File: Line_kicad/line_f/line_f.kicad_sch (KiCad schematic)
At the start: 15 parts, among them M2 Motor_DC, M3 Motor_DC, SW1 SW_SPST, SW2 SW_SPDT, SW3 SW_Push, SW4 SW_Push, U1 TB6612FNG_LINE, m1 BLACKPILL

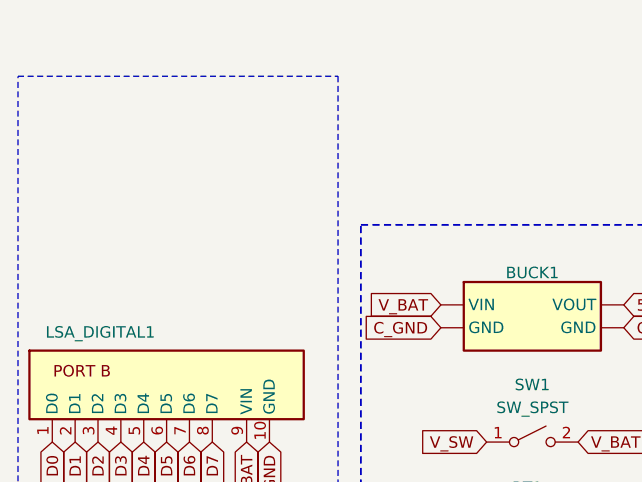
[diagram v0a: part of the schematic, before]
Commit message: 3#
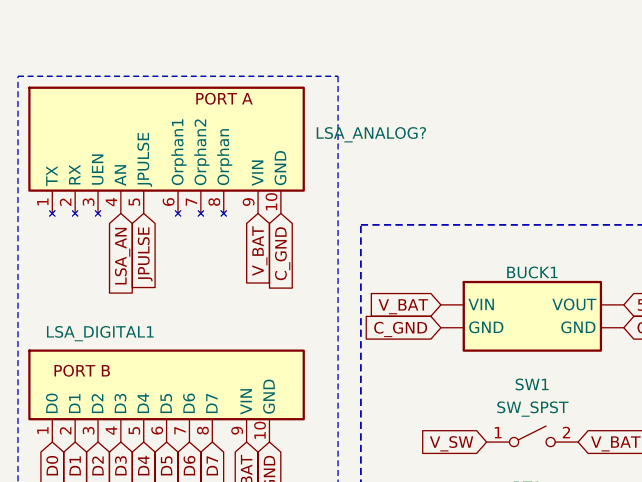
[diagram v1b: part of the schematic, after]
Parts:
- added LSA_ANALOG?: ~, symbol LINE_F_SYM_LIB:LSA_ANALOG
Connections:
- net C_GND: now also LSA_ANALOG?.10 (GND)
- net JPULSE: now also LSA_ANALOG?.5 (JPULSE)
- net LSA_AN: now also LSA_ANALOG?.4 (AN)
- net V_BAT: now also LSA_ANALOG?.9 (VIN)
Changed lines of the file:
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@@
+		)
+	)
+	(global_label "LSA_AN"
+		(shape input)
+		(at 36.83 83.82 270)
+		(fields_autoplaced yes)
+		(effects
+			(font
+				(size 1.27 1.27)
+			)
+			(justify right)
+		)
+		(property "Intersheetrefs" "${INTERSHEET_REFS}"
+			(at 36.83 93.5181 90)
+			(effects
+				(font
+					(size 1.27 1.27)
+				)
+				(justify right)
+				(hide yes)
+			)
+		)
+	)
+	(global_label "V_BAT"
+		(shape input)
+		(at 52.07 83.82 270)
+		(fields_autoplaced yes)
+		(effects
+			(font
+				(size 1.27 1.27)
+			)
+			(justify right)
+		)
+		(property "Intersheetrefs" "${INTERSHEET_REFS}"
+			(at 52.07 92.1876 90)
+			(effects
+				(font
+					(size 1.27 1.27)
+				)
+				(justify right)
+				(hide yes)
+			)
 		)
 	)
@@
 		)
 	)
+	(global_label "C_GND"
+		(shape input)
+		(at 54.61 83.82 270)
+		(fields_autoplaced yes)
+		(effects
+			(font
+				(size 1.27 1.27)
+			)
+			(justify right)
+		)
+		(property "Intersheetrefs" "${INTERSHEET_REFS}"
+			(at 54.61 92.9133 90)
+			(effects
+				(font
+					(size 1.27 1.27)
+				)
+				(justify right)
+				(hide yes)
+			)
+		)
+	)
 	(global_label "PWMA"
 		(shape input)
@@
 		)
 	)
+	(global_label "JPULSE"
+		(shape input)
+		(at 39.37 83.82 270)
+		(fields_autoplaced yes)
+		(effects
+			(font
+				(size 1.27 1.27)
+			)
+			(justify right)
+		)
+		(property "Intersheetrefs" "${INTERSHEET_REFS}"
+			(at 39.37 93.7599 90)
+			(effects
+				(font
+					(size 1.27 1.27)
+				)
+				(justify right)
+				(hide yes)
+			)
+		)
+	)
 	(global_label "D2"
 		(shape input)
@@
 			)
 		)
+	)
+	(symbol
+		(lib_id "LINE_F_SYM_LIB:LSA_ANALOG")
+		(at 41.91 78.74 0)
+		(unit 1)
+		(exclude_from_sim no)
+		(in_bom yes)
+		(on_board yes)
+		(dnp no)
+		(fields_autoplaced yes)
+		(property "Reference" "LSA_ANALOG?"
+			(at 58.42 74.9299 0)
+			(effects
+				(font
+					(size 1.27 1.27)
+				)
+				(justify left)
+			)
+		)
+		(property "Value" "~"
+			(at 58.42 76.835 0)
+			(effects
+				(font
+					(size 1.27 1.27)
+				)
+				(justify left)
+			)
+		)
+		(property "Footprint" ""
+			(at 41.91 78.74 0)
+			(effects
+				(font
+					(size 1.27 1.27)
+				)
+				(hide yes)
+			)
+		)
+		(property "Datasheet" ""
+			(at 41.91 78.74 0)
+			(effects
+				(font
+					(size 1.27 1.27)
+				)
+				(hide yes)
+			)
+		)
+		(property "Description" ""
+			(at 41.91 78.74 0)
+			(effects
+				(font
+					(size 1.27 1.27)
+				)
+				(hide yes)
+			)
+		)
+		(pin "1"
+		)
+		(pin "5"
+		)
+		(pin "9"
+		)
+		(pin "7"
+		)
+		(pin "2"
+		)
+		(pin "10"
+		)
+		(pin "3"
+		)
+		(pin "6"
+		)
+		(pin "4"
+		)
+		(pin "8"
+		)
+		(instances
+			(project ""
+				(path "/c13c4e87-a023-4a7d-8b82-fe1a380f0003"
+					(reference "LSA_ANALOG?")
+					(unit 1)
+				)
+			)
+		)

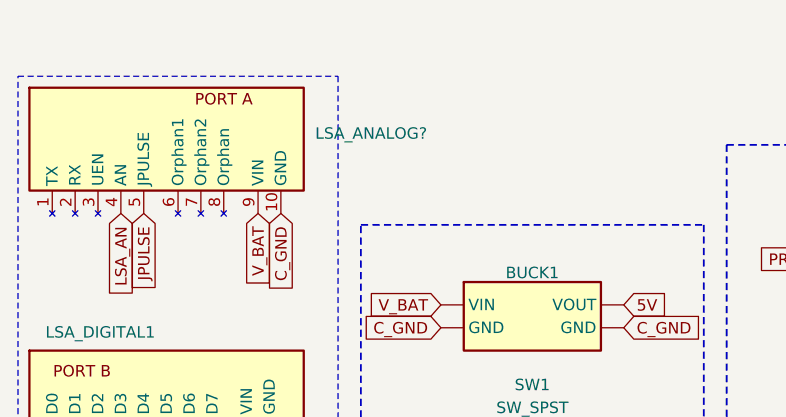
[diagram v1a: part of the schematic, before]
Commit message: 4#
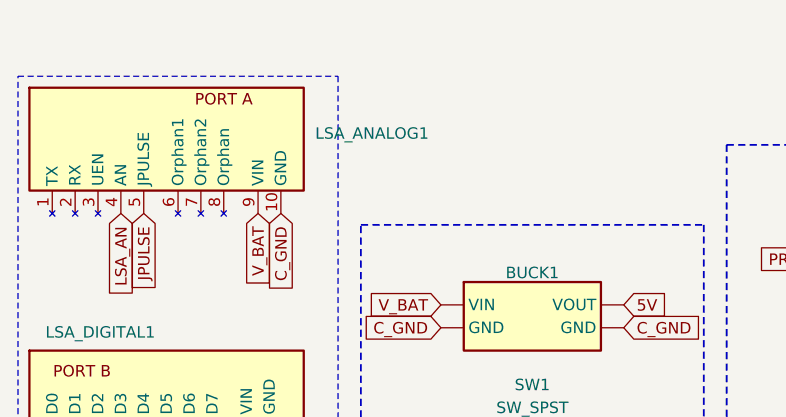
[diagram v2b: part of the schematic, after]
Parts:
- gave numbers to parts that had none: 1
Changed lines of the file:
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@@
 		(dnp no)
 		(fields_autoplaced yes)
-		(property "Reference" "LSA_ANALOG?"
+		(property "Reference" "LSA_ANALOG1"
 			(at 58.42 74.9299 0)
 			(effects
@@
 			(project ""
 				(path "/c13c4e87-a023-4a7d-8b82-fe1a380f0003"
-					(reference "LSA_ANALOG?")
+					(reference "LSA_ANALOG1")
 					(unit 1)
 				)

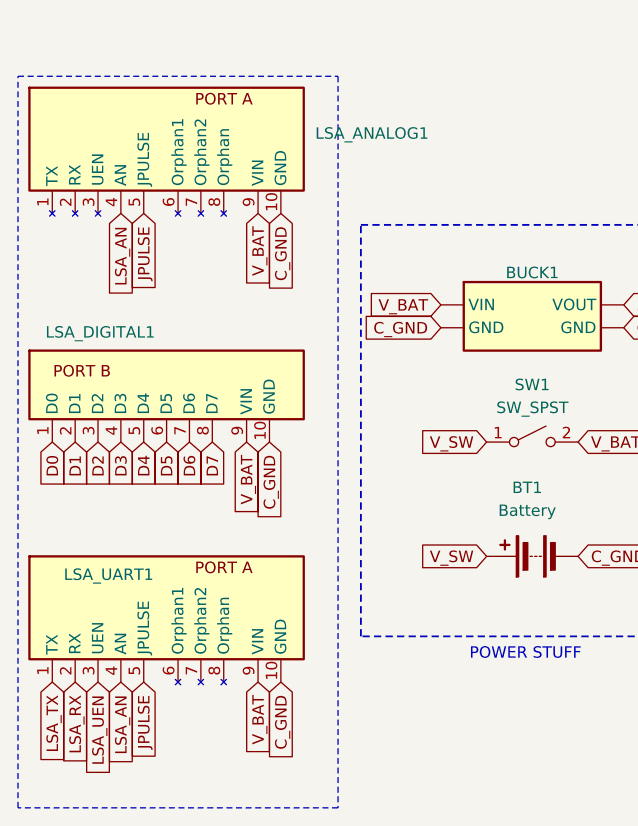
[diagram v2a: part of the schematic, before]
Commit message: 4#
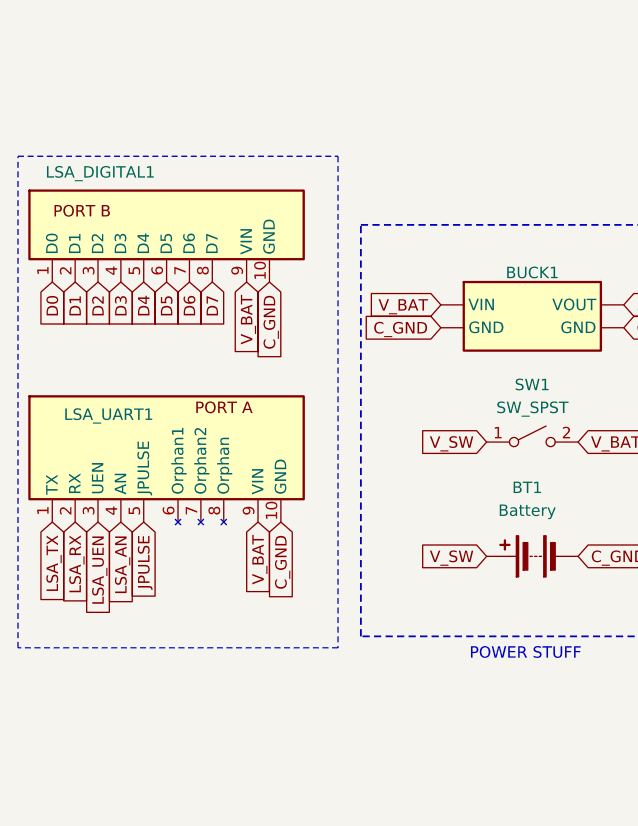
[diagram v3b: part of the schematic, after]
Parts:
- removed LSA_ANALOG1: ~, symbol LINE_F_SYM_LIB:LSA_ANALOG
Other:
- moved on the sheet: LSA_DIGITAL1, LSA_UART1

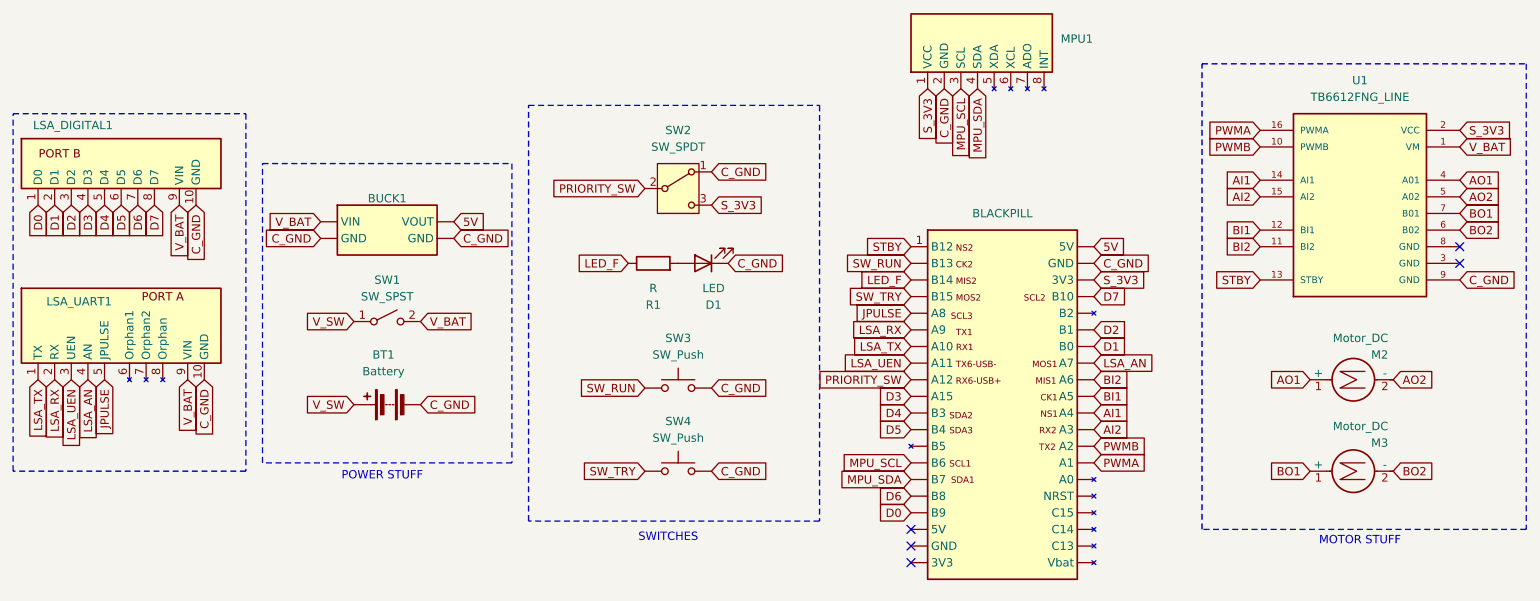
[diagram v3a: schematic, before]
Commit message: 4#
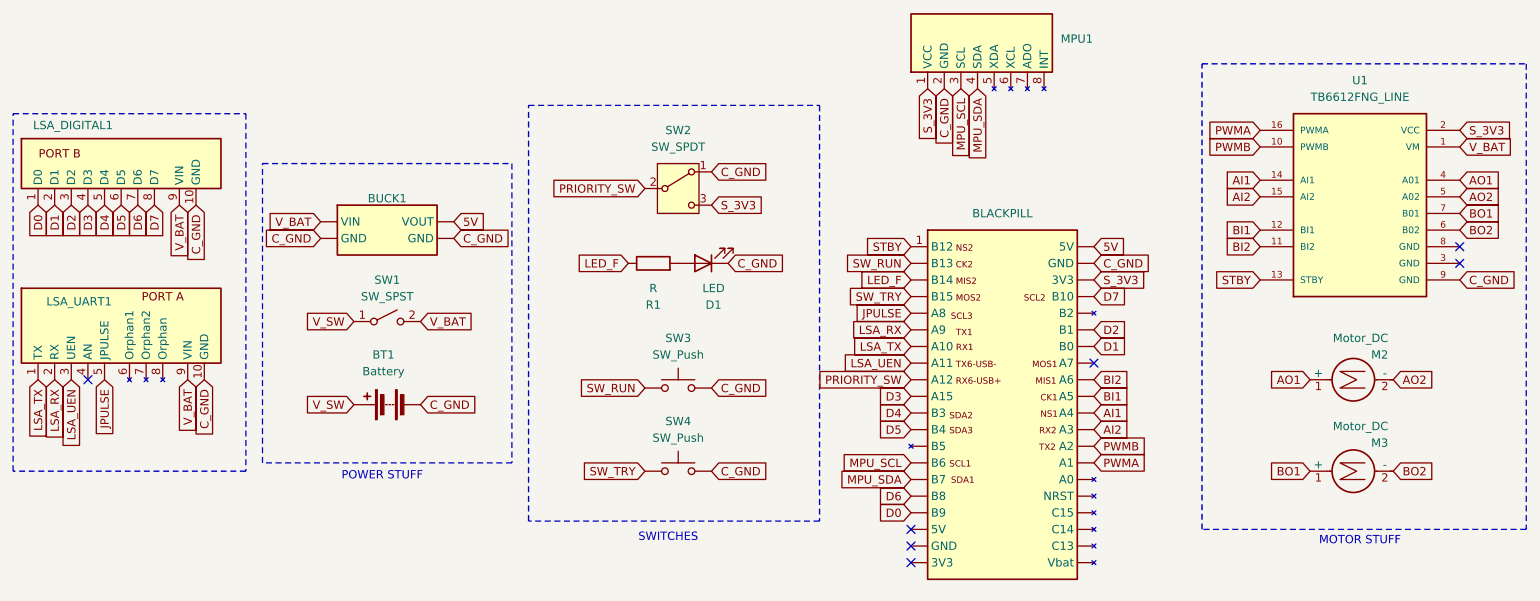
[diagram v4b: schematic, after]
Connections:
- net LSA_AN: no longer names the net of m1.28 (A7)
- net LSA_AN: no longer LSA_UART1.4 (AN)
- no-connect marks 5 -> 7
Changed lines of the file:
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@@
 	(paper "A4")
 	(no_connect
+		(at 36.83 118.11)
+	)
+	(no_connect
 		(at 162.56 143.51)
+	)
+	(no_connect
+		(at 190.5 115.57)
 	)
 	(no_connect
@@
 		)
 	)
-	(global_label "LSA_AN"
-		(shape input)
-		(at 190.5 115.57 0)
-		(fields_autoplaced yes)
-		(effects
-			(font
-				(size 1.27 1.27)
-			)
-			(justify left)
-		)
-		(property "Intersheetrefs" "${INTERSHEET_REFS}"
-			(at 200.1981 115.57 0)
-			(effects
-				(font
-					(size 1.27 1.27)
-				)
-				(justify left)
-				(hide yes)
-			)
-		)
-	)
 	(global_label "C_GND"
 		(shape input)
@@
 			(effects
 				(font
-					(size 1.27 1.27)
-				)
-				(justify right)
-				(hide yes)
-			)
-		)
-	)
-	(global_label "LSA_AN"
-		(shape input)
-		(at 36.83 118.11 270)
-		(fields_autoplaced yes)
-		(effects
-			(font
-				(size 1.27 1.27)
-			)
-			(justify right)
-		)
-		(property "Intersheetrefs" "${INTERSHEET_REFS}"
-			(at 36.83 127.8081 90)
-			(effects
-				(font

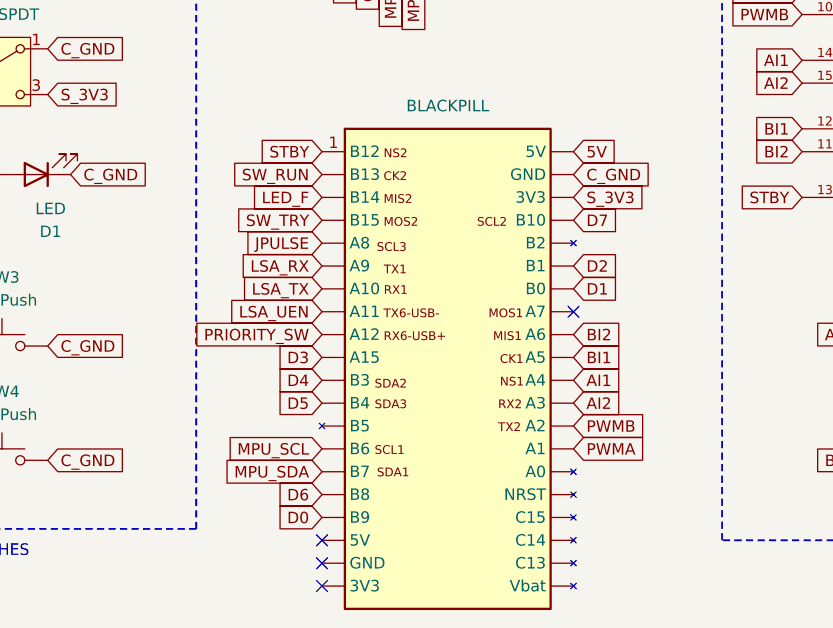
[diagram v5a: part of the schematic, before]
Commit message: 5#
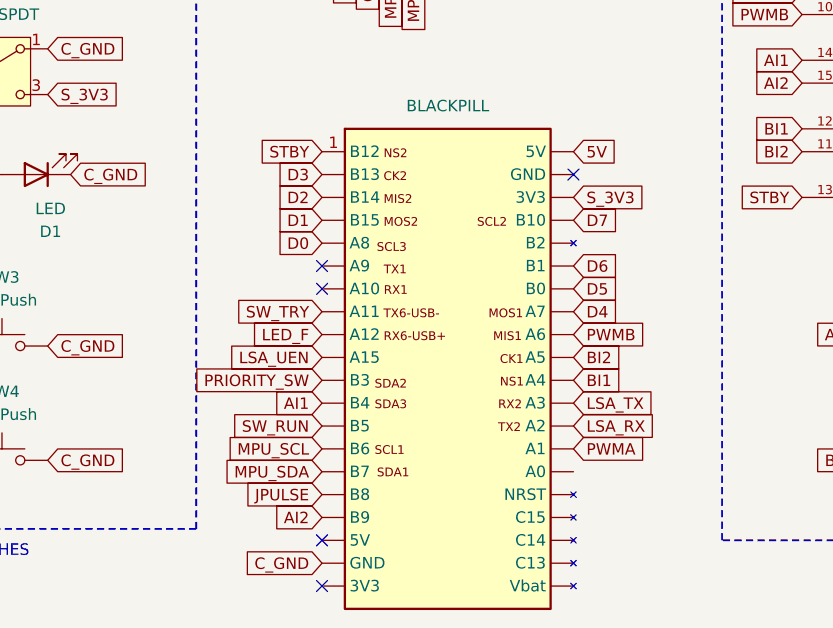
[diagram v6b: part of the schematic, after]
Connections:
- net AI1: now also m1.12 (B4); no longer m1.31 (A4)
- net AI2: now also m1.17 (B9); no longer m1.32 (A3)
- net BI1: now also m1.31 (A4); no longer m1.30 (A5)
- net BI2: now also m1.30 (A5); no longer m1.29 (A6)
- net C_GND: now also m1.19 (GND); no longer m1.22 (GND)
- net D0: now also m1.5 (A8); no longer m1.17 (B9)
- net D1: now also m1.4 (B15); no longer m1.27 (B0)
- net D2: now also m1.3 (B14); no longer m1.26 (B1)
- net D3: now also m1.2 (B13); no longer m1.10 (A15)
- net D4: now also m1.28 (A7); no longer m1.11 (B3)
- net D5: now also m1.27 (B0); no longer m1.12 (B4)
- net D6: now also m1.26 (B1); no longer m1.16 (B8)
- net JPULSE: now also m1.16 (B8); no longer m1.5 (A8)
- net LED_F: now also m1.9 (A12); no longer m1.3 (B14)
- net LSA_RX: now also m1.33 (A2); no longer m1.6 (A9)
- net LSA_TX: now also m1.32 (A3); no longer m1.7 (A10)
- net LSA_UEN: now also m1.10 (A15); no longer m1.8 (A11)
- net PRIORITY_SW: now also m1.11 (B3); no longer m1.9 (A12)
- net PWMB: now also m1.29 (A6); no longer m1.33 (A2)
- net SW_RUN: now also m1.13 (B5); no longer m1.2 (B13)
- net SW_TRY: now also m1.8 (A11); no longer m1.4 (B15)
- no-connect marks 7 -> 8

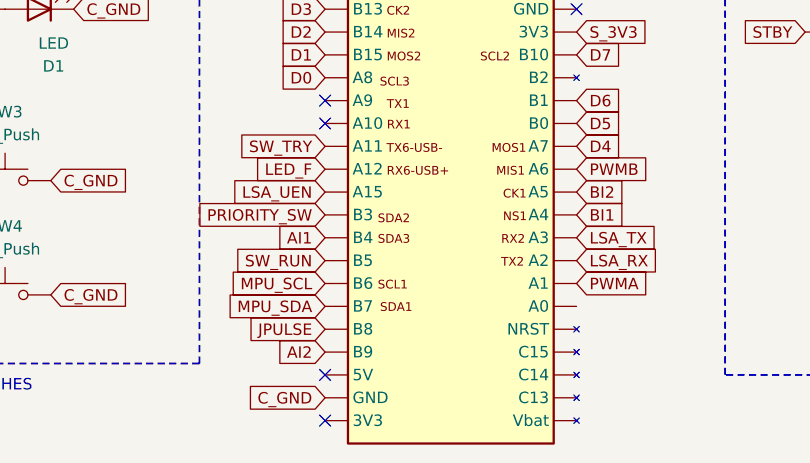
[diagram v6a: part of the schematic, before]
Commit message: pin1
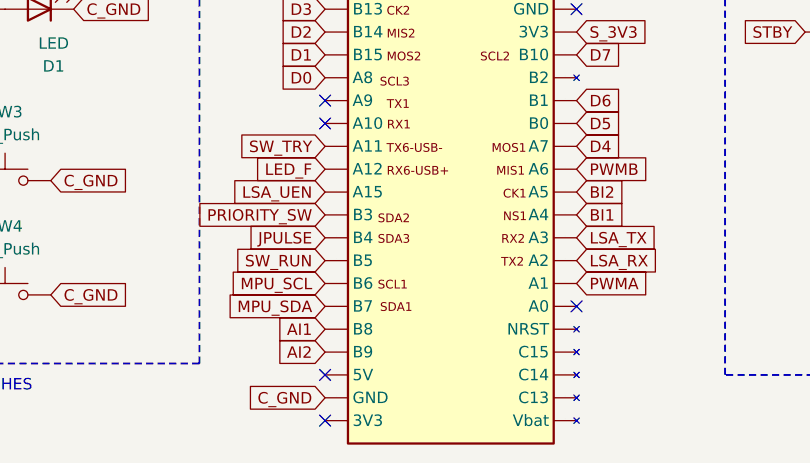
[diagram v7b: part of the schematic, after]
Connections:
- net AI1: now also m1.16 (B8); no longer m1.12 (B4)
- net JPULSE: now also m1.12 (B4); no longer m1.16 (B8)
- no-connect marks 8 -> 9

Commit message: pin1
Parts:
- U1: footprint LINE_F_FOOT_LIB:TB6612FNG_LINE -> ROB-14450:MODULE_ROB-14450
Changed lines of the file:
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@@
+			)
+		)
+		(property "Sim.Pins" "1=K 2=A"
+			(at 130.81 100.33 0)
+			(effects
+				(font
+					(size 1.27 1.27)
+				)
+				(hide yes)
 			)
 		)
@@
 			)
 		)
-		(property "Footprint" "LINE_F_FOOT_LIB:TB6612FNG_LINE"
+		(property "Footprint" "ROB-14450:MODULE_ROB-14450"
 			(at 231.14 92.71 0)
 			(effects
